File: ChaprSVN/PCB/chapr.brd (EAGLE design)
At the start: 70.9 x 54.1 mm, 20 parts, among them M2 RN42 Module

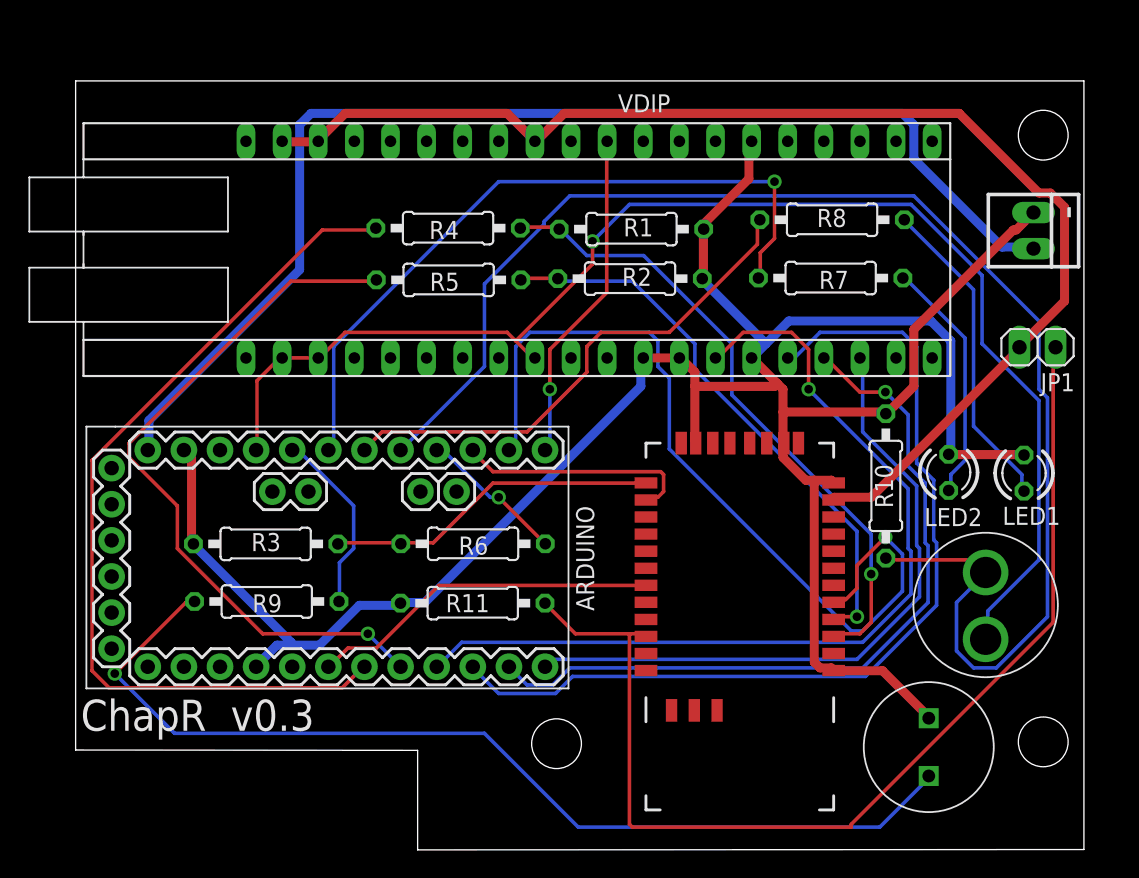
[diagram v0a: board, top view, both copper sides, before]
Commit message: Intermediate version with new power-on circuit.  NOT COMPLETE.
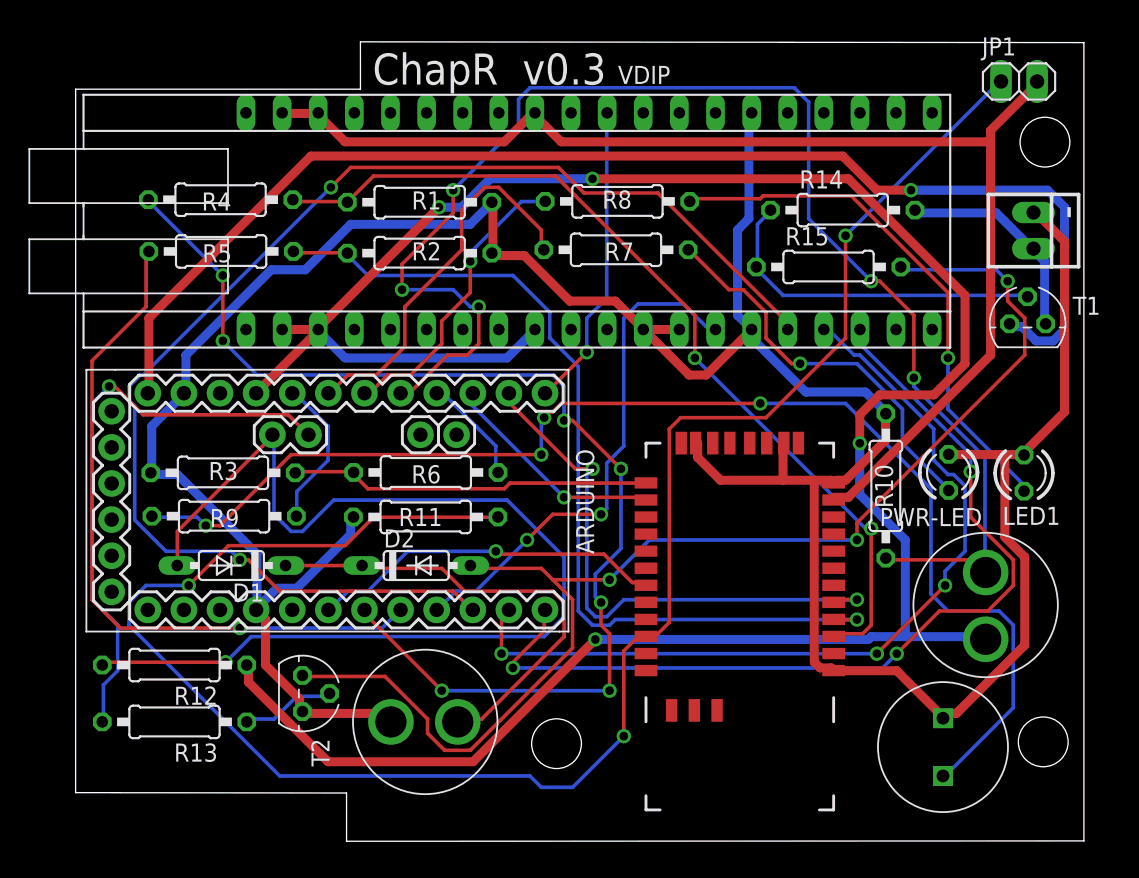
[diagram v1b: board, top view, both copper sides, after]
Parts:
- added D1, D2: 1N4148, diode:DO35-7
- added PB2: BUTTON, ChapR-Custom:2-PIN-PUSHBUTTON
- added R12, R13, R15: 12k, resistor:0207/10
- added R14: 22k, resistor:0207/10
- added T1, T2: (no value), transistor:TO92
- moved JP1 18.7 mm to (66.4, 54.0), turned to 0 degrees
- moved R5 16.1 mm to (10.3, 42.1)
- moved R4 16.1 mm to (10.2, 45.7)
- moved R7 15.2 mm to (38.1, 42.2)
- moved R8 15.2 mm to (38.2, 45.6)
- moved R1 15.0 mm to (24.2, 45.6)
- moved R2 14.9 mm to (24.2, 42.0)
- moved R11 6.91 mm to (24.7, 23.4)
- moved R9 6.71 mm to (10.5, 23.5)
- moved R6 6.02 mm to (24.7, 26.5)
- moved R3 5.83 mm to (10.4, 26.5)
- moved ARDUINO 4.00 mm to (17.8, 25.8)
- moved VDIP 2.00 mm to (36.2, 44.2)
- moved U$2 1.00 mm to (61.0, 7.23)
- renumbered LED2 to PWR-LED
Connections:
- net 3.3V renamed +3V3
- new net +5V: ARDUINO.VCC, PB1.P$1, R12.1, VDIP.2, VDIP.3, VDIP.9
- new net N$23: ARDUINO.RAWV, T1.3
- new net N$25: D2.A, R15.2, T2.3
- new net N$26: R13.1, T2.2
- new net N$27: D1.C, D2.C, PB2.P$2
- new net N$29: ARDUINO.A5, D1.A, R12.2
- new net N$30: ARDUINO.A4, R13.2
- net +9V: now also R14.2, T1.1; no longer ARDUINO.RAWV
- net GND: now also PB2.P$1, T2.1
- net N$1: now also R14.1, R15.1, T1.2; no longer ARDUINO.VCC, PB1.P$1, VDIP.2, VDIP.3, VDIP.9
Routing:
- net +5V: track 0.00 -> 168.9 mm, vias 0 -> 4
- net N$25: track 0.00 -> 90.4 mm, vias 0 -> 3
- net N$23: track 0.00 -> 89.3 mm, vias 0 -> 1
- net N$29: track 0.00 -> 79.2 mm, vias 0 -> 1
- net N$1: track 95.2 -> 24.4 mm, vias 1 -> 0
- net +9V: track 84.6 -> 15.2 mm
- net N$22: track 76.9 -> 132.4 mm, vias 0 -> 3
- net GND: track 176.5 -> 222.9 mm
- net N$30: track 0.00 -> 40.7 mm, vias 0 -> 1
- net N$27: track 0.00 -> 33.2 mm
- net N$12: track 65.0 -> 93.6 mm, vias 0 -> 2
- net N$13: track 63.4 -> 36.5 mm, vias 1 -> 2
- net N$18: track 50.5 -> 26.9 mm, vias 1 -> 0
- net N$7: track 40.0 -> 63.5 mm
- net N$14: track 61.8 -> 81.9 mm, vias 0 -> 7
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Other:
- board size 70.9 x 54.1 mm -> 70.9 x 56.2 mm
